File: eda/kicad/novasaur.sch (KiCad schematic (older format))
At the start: 30 parts, among them J9 RAM, SW1 RESET, U1 74F86, U10 74F574, U11 74F574, U12 ATF16V8B, U2 74F08, U3 74F32, U4 74ALS139, U5 74ALS139, U6 74F157, U7 74F175, U8 74F574, U9 74F138, X1 33M

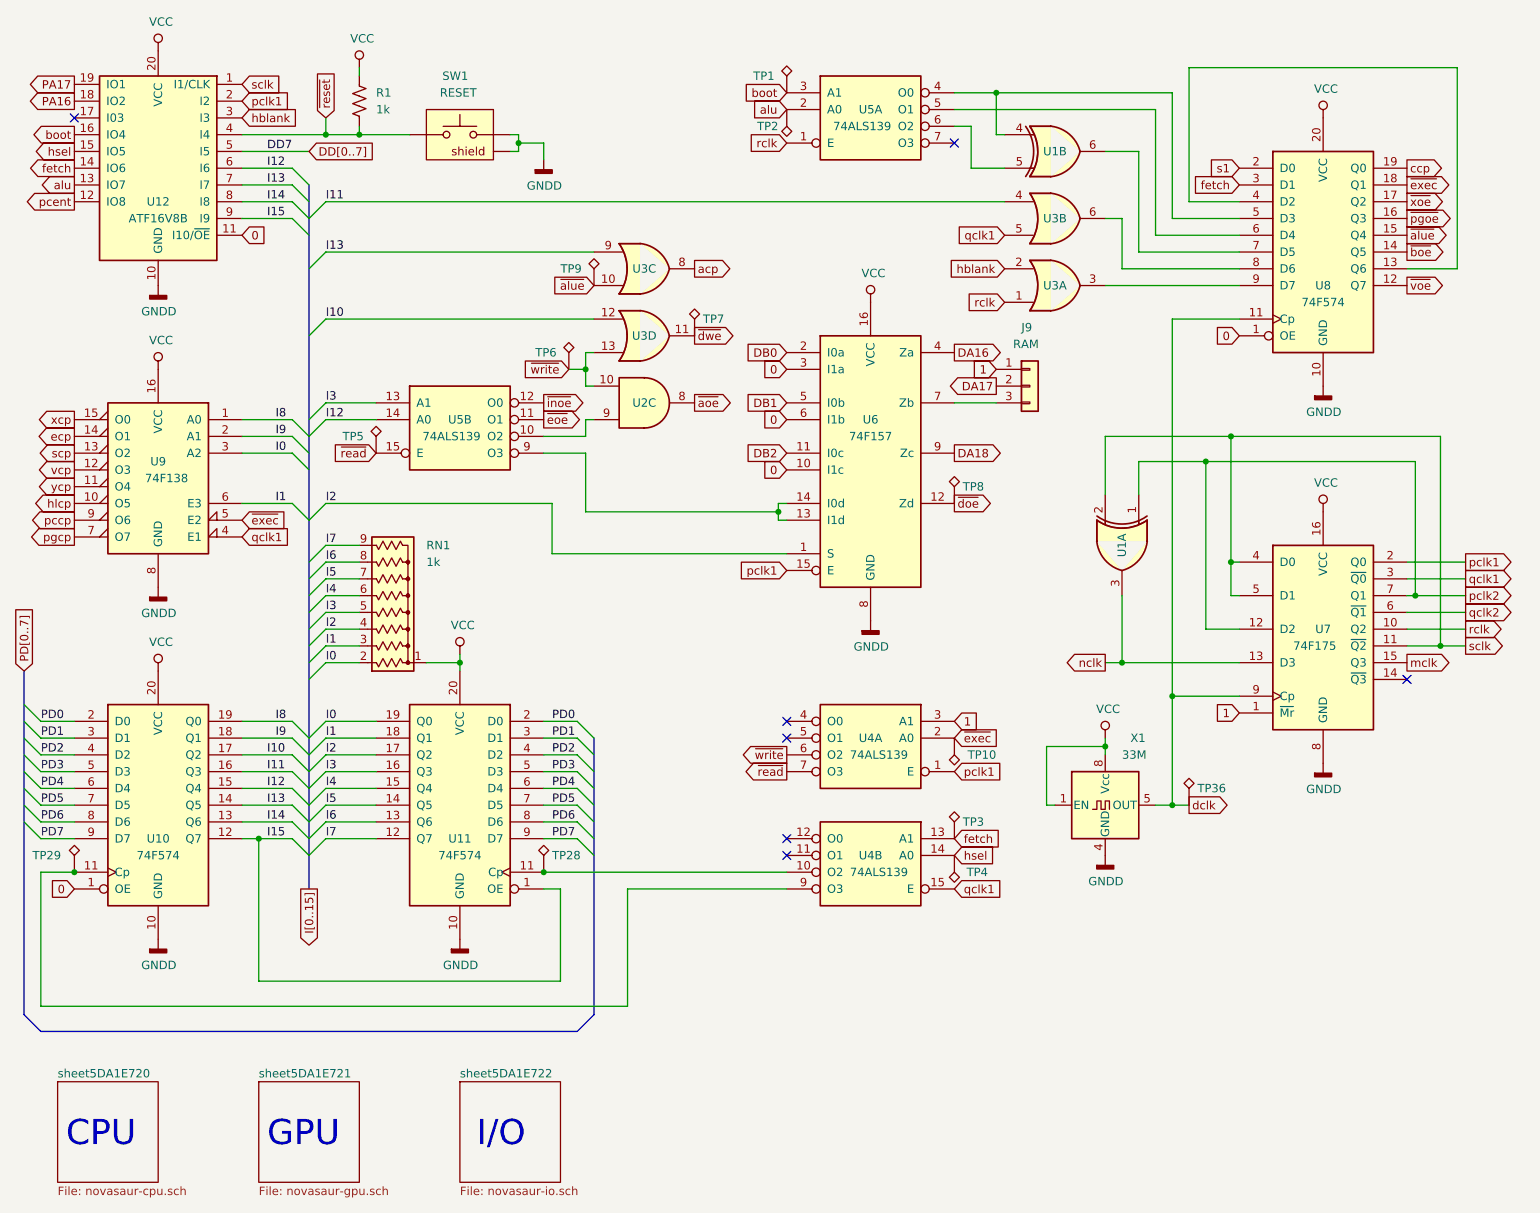
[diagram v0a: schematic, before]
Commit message: power sw + super caps
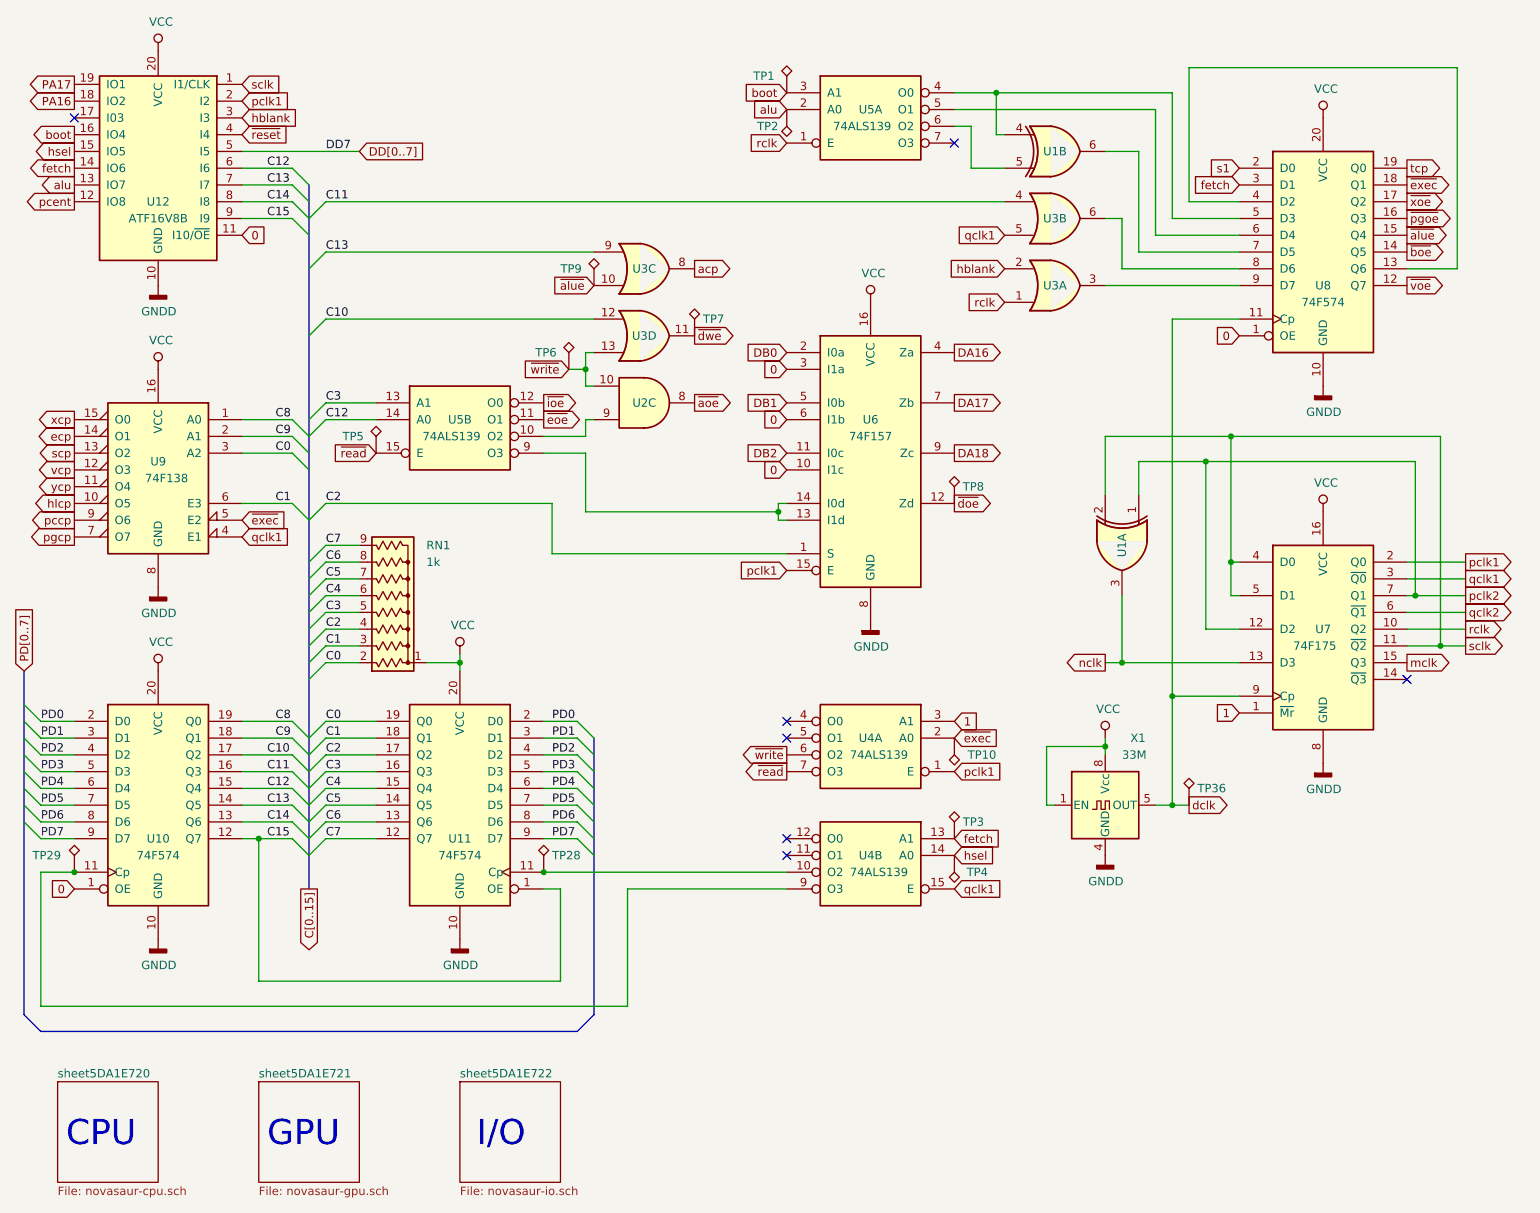
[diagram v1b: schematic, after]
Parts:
- removed J9: RAM, Connector_PinHeader_2.54mm:PinHeader_1x03_P2.54mm_Vertical, symbol Connector_Generic:Conn_01x03
- removed R1: 1k, Resistor_THT:R_Axial_DIN0204_L3.6mm_D1.6mm_P7.62mm_Horizontal, symbol Device:R_US
- removed SW1: RESET, FSMRA3JH04:SWITCH_FSMRA3JH04, symbol novasaur-rescue:SW_Push-Switch
- TP28: value ILCP -> CLCP
- TP29: value IHCP -> CHCP
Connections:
- net DA17: now also U6.7 (Zb)
- net I0 renamed C0
- net I1 renamed C1
- net I10 renamed C10
- net I11 renamed C11
- net I12 renamed C12
- net I13 renamed C13
- net I14 renamed C14
- net I15 renamed C15
- net I2 renamed C2
- net I3 renamed C3
- net I4 renamed C4
- net I5 renamed C5
- net I6 renamed C6
- net I7 renamed C7
- net I8 renamed C8
- net I9 renamed C9
- net ccp renamed tcp
- net ~inoe renamed ~ioe
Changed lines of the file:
@@
 Sheet 1 4
 Title "Novasaur Retrocomputer"
-Date "2020-03-31"
+Date "2020-05-02"
 Rev "1.6"
 Comp ""
@@
 Wire Wire Line
 	4250 6000 4250 6550
-$Comp
-L novasaur-rescue:SW_Push-Switch SW1
-U 1 1 5E0603B4
-P 3650 1500
-AR Path="/5E0603B4" Ref="SW1"  Part="1"
-AR Path="/5CDEEC9F/5E0603B4" Ref="SW?"  Part="1"
-AR Path="/62D13D9D/5E0603B4" Ref="SW?"  Part="1"
-AR Path="/5DAA5CD8/5E0603B4" Ref="SW?"  Part="1"
-F 0 "SW1" H 3600 1850 50  0000 L CNN
-F 1 "RESET" H 3550 1750 50  0000 L CNN
-F 2 "FSMRA3JH04:SWITCH_FSMRA3JH04" H 3650 1700 50  0001 C CNN
-F 3 "~" H 3650 1700 50  0001 C CNN
-	1    3650 1500
-	-1   0    0    -1
-$EndComp
 Text GLabel 1350 1800 0    50   Output ~ 0
 alu
@@
 pcent
 Text Label 2500 1700 0    50   ~ 0
-I12
+C12
 Entry Wire Line
 	2650 1700 2750 1800
-Text GLabel 2750 1600 2    50   Input ~ 0
+Text GLabel 3050 1600 2    50   Input ~ 0
 DD[0..7]
 Wire Wire Line
@@
 $EndComp
 Text Label 2550 3200 0    50   ~ 0
-I8
+C8
 Text Label 2550 3300 0    50   ~ 0
-I9
+C9
 Text Label 2550 3400 0    50   ~ 0
-I0
+C0
 Text Label 2500 1900 0    50   ~ 0
-I14
+C14
 Text GLabel 2750 6000 3    50   Output ~ 0
-I[0..15]
+C[0..15]
 Entry Wire Line
 	2650 3200 2750 3300
@@
 	4450 5800 4350 5700
 Text Label 2550 5000 0    50   ~ 0
-I8
+C8
 Text Label 2550 5100 0    50   ~ 0
-I9
+C9
 Text Label 2500 5200 0    50   ~ 0
-I10
+C10
 Text Label 2500 5300 0    50   ~ 0
-I11
+C11
 Text Label 2500 5400 0    50   ~ 0
-I12
+C12
 Text Label 2500 5500 0    50   ~ 0
-I13
+C13
 Text Label 2500 5600 0    50   ~ 0
-I14
+C14
 Text Label 2500 5700 0    50   ~ 0
-I15
+C15
 Text Label 4200 5000 0    50   ~ 0
 PD0
@@
 	2650 1900 2750 2000
 Text Label 2500 1800 0    50   ~ 0
-I13
+C13
 Entry Wire Line
 	2650 1800 2750 1900
@@
 PD0
 Text Label 2850 5700 0    50   ~ 0
-I7
+C7
 Text Label 2850 5600 0    50   ~ 0
-I6
+C6
 Text Label 2850 5500 0    50   ~ 0
-I5
+C5
 Text Label 2850 5400 0    50   ~ 0
-I4
+C4
 Text Label 2850 5300 0    50   ~ 0
-I3
+C3
 Text Label 2850 5200 0    50   ~ 0
-I2
+C2
 Text Label 2850 5100 0    50   ~ 0
-I1
+C1
 Text Label 2850 5000 0    50   ~ 0
-I0
+C0
 Entry Wire Line
 	2750 5800 2650 5700
@@
 	1150 5000 1050 4900
 Text Label 2550 3700 0    50   ~ 0
-I1
+C1
 Text GLabel 1350 3900 0    50   Output ~ 0
 pgcp
@@
 $EndComp
 Text Label 2500 2000 0    50   ~ 0
-I15
+C15
 Entry Wire Line
 	2750 4650 2850 4550
@@
 	2850 4650 3050 4650
 Text Label 2850 4650 0    50   ~ 0
-I0
+C0
 Text Label 2850 4550 0    50   ~ 0
-I1
+C1
 Text Label 2850 4450 0    50   ~ 0
-I2
+C2
 Text Label 2850 4350 0    50   ~ 0
-I3
+C3
 Text Label 2850 4250 0    50   ~ 0
-I4
+C4
 Text Label 2850 4150 0    50   ~ 0
-I5
+C5
 Text Label 2850 4050 0    50   ~ 0
-I6
+C6
 Text Label 2850 3950 0    50   ~ 0
-I7
+C7
 $Comp
 L power:VCC #PWR?
@@
 ~exec
 Text GLabel 9300 1700 2    50   Output ~ 0
-ccp
+tcp
 Text GLabel 6900 2300 0    50   Input ~ 0
 hblank
@@
 	1    0    0    -1
 $EndComp
-$Comp
-L power:GNDD #PWR?
-U 1 1 5DEF95A1
-P 4150 1650
-AR Path="/5CDEEC9F/5DEF95A1" Ref="#PWR?"  Part="1"
-AR Path="/5DAA5CD8/5DEF95A1" Ref="#PWR?"  Part="1"
-AR Path="/5DEF95A1" Ref="#PWR0194"  Part="1"
-F 0 "#PWR0194" H 4150 1400 50  0001 C CNN
-F 1 "GNDD" H 4154 1495 50  0000 C CNN
-F 2 "" H 4150 1650 50  0001 C CNN
-F 3 "" H 4150 1650 50  0001 C CNN
-	1    4150 1650
-	1    0    0    -1
-$EndComp
-Wire Wire Line
-	4150 1550 4150 1650
-Wire Wire Line
-	4000 1600 4000 1550
-Wire Wire Line
-	4000 1500 3950 1500
-Wire Wire Line
-	4000 1550 4150 1550
-Connection ~ 4000 1550
-Wire Wire Line
-	4000 1550 4000 1500
-Text Label 2500 1600 0    50   ~ 0
+Text Label 2850 1600 0    50   ~ 0
 DD7
-$Comp
-L Device:R_US R?
-U 1 1 5E523FD1
-P 3050 1300
-AR Path="/62D13D9D/5E523FD1" Ref="R?"  Part="1"
-AR Path="/5DAA19D5/5E523FD1" Ref="R?"  Part="1"
-AR Path="/5DAA5CD8/5D99DA9F/5E523FD1" Ref="R?"  Part="1"
-AR Path="/5DA1E9BA/5E523FD1" Ref="R?"  Part="1"
-AR Path="/5E523FD1" Ref="R1"  Part="1"
-F 0 "R1" H 3150 1350 50  0000 L CNN
-F 1 "1k" H 3150 1250 50  0000 L CNN
-F 2 "Resistor_THT:R_Axial_DIN0204_L3.6mm_D1.6mm_P7.62mm_Horizontal" V 3090 1290 50  0001 C CNN
-F 3 "~" H 3050 1300 50  0001 C CNN
-	1    3050 1300
-	1    0    0    -1
-$EndComp
-$Comp
-L power:VCC #PWR?
-U 1 1 5E54FDAD
-P 3050 1100
-AR Path="/5CDEEC9F/5E54FDAD" Ref="#PWR?"  Part="1"
-AR Path="/5DAA5CD8/5E54FDAD" Ref="#PWR?"  Part="1"
-AR Path="/5E54FDAD" Ref="#PWR0111"  Part="1"
-F 0 "#PWR0111" H 3050 950 50  0001 C CNN
-F 1 "VCC" H 3067 1273 50  0000 C CNN
-F 2 "" H 3050 1100 50  0001 C CNN
-F 3 "" H 3050 1100 50  0001 C CNN
-	1    3050 1100
-	1    0    0    -1
-$EndComp
-Wire Wire Line
-	3050 1500 3050 1450
-Wire Wire Line
-	3050 1150 3050 1100
 Wire Wire Line
 	9600 1100 8000 1100
@@
 	2850 3200 3150 3200
 Text Label 2850 3100 0    50   ~ 0
-I3
+C3
 Text GLabel 3150 3400 0    50   Input ~ 0
 ~read
@@
 acp
 Text GLabel 4150 3100 2    50   Output ~ 0
-~inoe
+~ioe
 Entry Wire Line
 	2850 2200 2750 2300
 Text Label 2850 2200 0    50   ~ 0
-I13
+C13
 Text Label 2850 3200 0    50   ~ 0
-I12
+C12
 Entry Wire Line
 	2850 3100 2750 3200
@@
 $EndSheet
 Text Label 2850 3700 0    50   ~ 0
-I2
+C2
 Entry Wire Line
 	2850 3700 2750 3800
@@
 	2850 2600 2750 2700
 Text Label 2850 2600 0    50   ~ 0
-I10
+C10
 Wire Wire Line
 	2850 2600 4450 2600
@@
 	2850 1900 2750 2000
 Text Label 2850 1900 0    50   ~ 0
-I11
+C11
 Wire Wire Line
 	2850 2200 4450 2200
@@
 $EndComp
 Wire Wire Line
-	3950 1600 4000 1600
-Wire Wire Line
 	7600 4650 7500 4650
 Connection ~ 7600 4650
-Text GLabel 6850 3000 0    50   Output ~ 0
+Text GLabel 6600 3100 2    50   Output ~ 0
 DA17
 Wire Wire Line
@@
 	2850 3700 4200 3700
 Wire Wire Line
-	2750 1600 2350 1600
-Connection ~ 3050 1500
-Wire Wire Line
-	2350 1500 2850 1500
-Wire Wire Line
 	4200 3700 4200 4000
-$Comp
-L Connector_Generic:Conn_01x03 J?
-U 1 1 5E60D57E
-P 7050 3000
-AR Path="/5DA1E9C0/5E60D57E" Ref="J?"  Part="1"
-AR Path="/5E60D57E" Ref="J9"  Part="1"
-F 0 "J9" H 7000 3350 50  0000 L CNN
-F 1 "RAM" H 6950 3250 50  0000 L CNN
-F 2 "Connector_PinHeader_2.54mm:PinHeader_1x03_P2.54mm_Vertical" H 7050 3000 50  0001 C CNN
-F 3 "~" H 7050 3000 50  0001 C CNN
-	1    7050 3000
-	1    0    0    -1
-$EndComp
-Wire Wire Line
-	6600 3100 6850 3100
-Text GLabel 6850 2900 0    50   Input ~ 0
-1
 $Comp
 L Connector:TestPoint_Alt TP29
@@
 AR Path="/5DA1E9C0/5E51CAB2" Ref="TP?"  Part="1"
 F 0 "TP29" H 1100 6000 50  0000 L CNN
-F 1 "IHCP" H 1100 6050 50  0001 L CNN
+F 1 "CHCP" H 1100 6050 50  0001 L CNN
 F 2 "TestPoint:TestPoint_Pad_1.0x1.0mm" H 1550 5900 50  0001 C CNN
 F 3 "~" H 1550 5900 50  0001 C CNN
@@
 	5600 5900 4150 5900
 Connection ~ 4150 5900
-Text GLabel 2850 1400 1    50   Input ~ 0
+Text GLabel 2350 1500 2    50   Input ~ 0
 ~reset
-Wire Wire Line
-	3050 1500 3350 1500
-Wire Wire Line
-	2850 1400 2850 1500
-Connection ~ 2850 1500
-Wire Wire Line
-	2850 1500 3050 1500
-Wire Bus Line
-	4450 5100 4450 6750
-Wire Bus Line
-	1050 4700 1050 6750
-Wire Bus Line
-	2750 1800 2750 6000
 $Comp
 L Connector:TestPoint_Alt TP28
@@
 AR Path="/5DA1E9C0/5E514E07" Ref="TP?"  Part="1"
 F 0 "TP28" H 4200 6000 50  0000 L CNN
-F 1 "ILCP" H 3900 6050 50  0001 L CNN
+F 1 "CLCP" H 3900 6050 50  0001 L CNN
 F 2 "TestPoint:TestPoint_Pad_1.0x1.0mm" H 4350 5900 50  0001 C CNN
 F 3 "~" H 4350 5900 50  0001 C CNN
@@
 	1    0    0    -1
 $EndComp
+Wire Wire Line
+	2350 1600 3050 1600
+Wire Bus Line
+	4450 5100 4450 6750
+Wire Bus Line
+	1050 4700 1050 6750
+Wire Bus Line
+	2750 1800 2750 6000
 $EndSCHEMATC
